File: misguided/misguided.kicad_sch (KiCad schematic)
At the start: 4 parts, among them J101 Conn_01x03, J102 Conn_01x03, J103 Conn_01x03

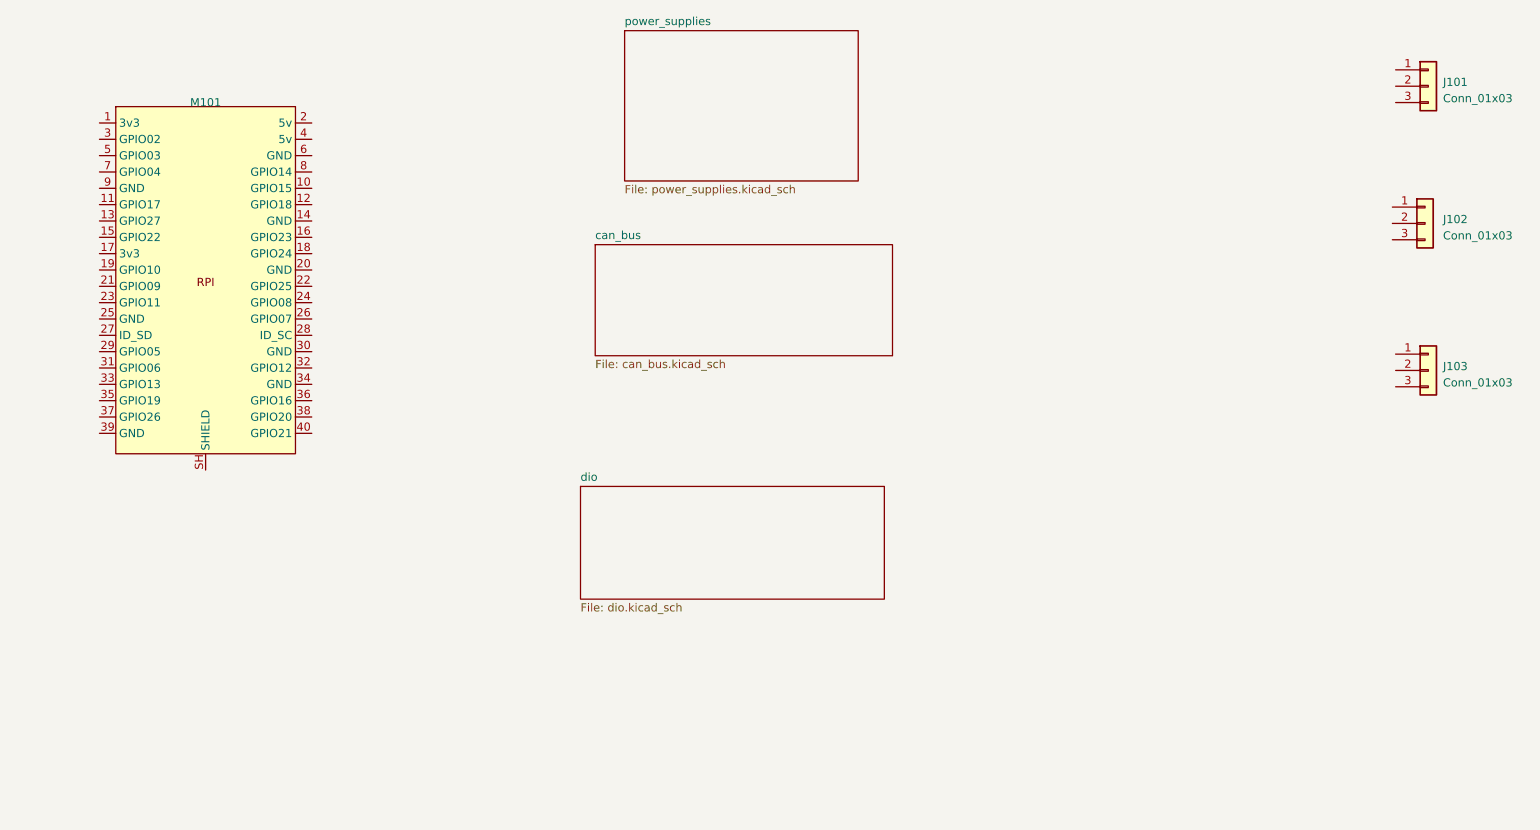
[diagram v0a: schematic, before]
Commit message: various fixes
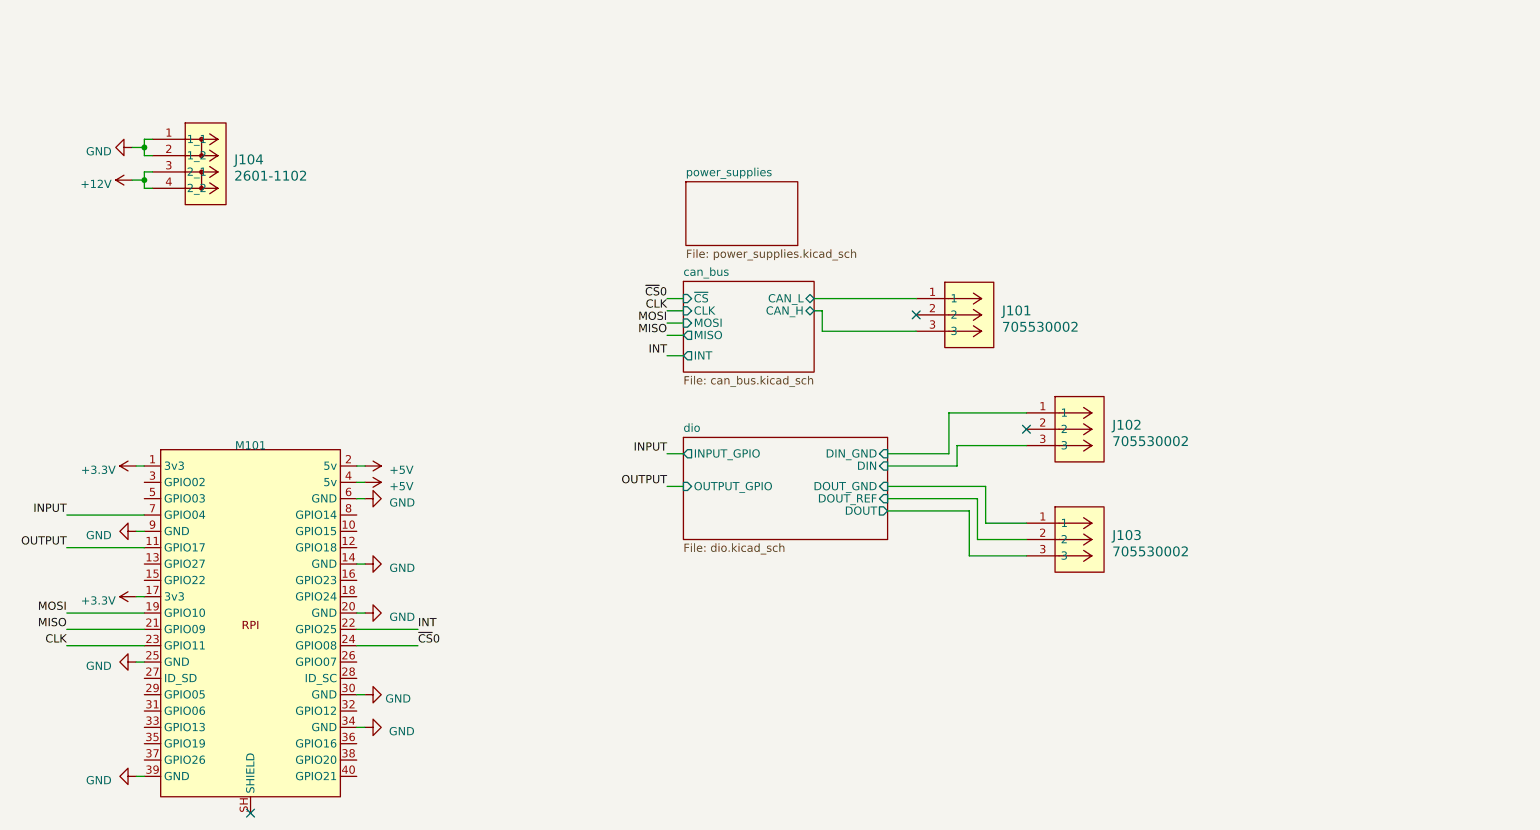
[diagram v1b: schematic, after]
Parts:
- removed J101, J102, J103: Conn_01x03, symbol Connector_Generic:Conn_01x03
- added J101, J102, J103: 705530002, CONN_705530002_03_MOL, symbol misguided:705530002
- added J104: 2601-1102, CONN2_2601-1102_WAG, symbol misguided:2601-1102
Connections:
- net +3.3V: now reaches M101.1 (3v3)
- net +3.3V: now also M101.17 (3v3)
- net OUTPUT: now reaches M101.11 (GPIO17)
- net GND: now reaches M101.14 (GND)
- net GND: now also M101.20 (GND), M101.25 (GND), M101.30 (GND), M101.34 (GND), M101.39 (GND), M101.6 (GND), M101.9 (GND), J104.1 (1_1), J104.2 (1_2)
- net MOSI: now reaches M101.19 (GPIO10)
- net +5V: now reaches M101.2 (5v)
- net +5V: now also M101.4 (5v)
- net MISO: now reaches M101.21 (GPIO09)
- net INT: now reaches M101.22 (GPIO25)
- net CLK: now reaches M101.23 (GPIO11)
- net ~{CS}0: now reaches M101.24 (GPIO08)
- net INPUT: now reaches M101.7 (GPIO04)
- new net +12V: J104.3 (2_1), J104.4 (2_2)
- new net can_bus/CAN_H: J101.3
- new net can_bus/CAN_L: J101.1
- new net dio/DIN: J102.3
- new net dio/DIN_GND: J102.1
- new net dio/DOUT: J103.3
- new net dio/DOUT_GND: J103.1
- new net dio/DOUT_REF: J103.2
- no-connect marks 0 -> 3
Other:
- sheet can_bus ports: added CAN_H, CAN_L, CLK, INT, MISO, MOSI, ~{CS}; removed none
- sheet dio ports: added DIN, DIN_GND, DOUT, DOUT_GND, DOUT_REF, INPUT_GPIO, OUTPUT_GPIO; removed none
- moved on the sheet: M101
